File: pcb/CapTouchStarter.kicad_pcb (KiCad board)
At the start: 4 copper layers, 76.5 x 66 mm, 59 parts, among them J1 USB_C_Receptacle, J2 Conn_ARM_JTAG_SWD_10, J3 62684-50110, Q1 SS8050-G, Q2 SS8050-G, SW1 SW_SPDT, SW2 EN, SW3 BOOT, U1 CP2102N-A01-GQFN28, U2 BD48K33G-TLCT-ND, U3 ESP32-WROVER-E, U4 AMS1117-3.3

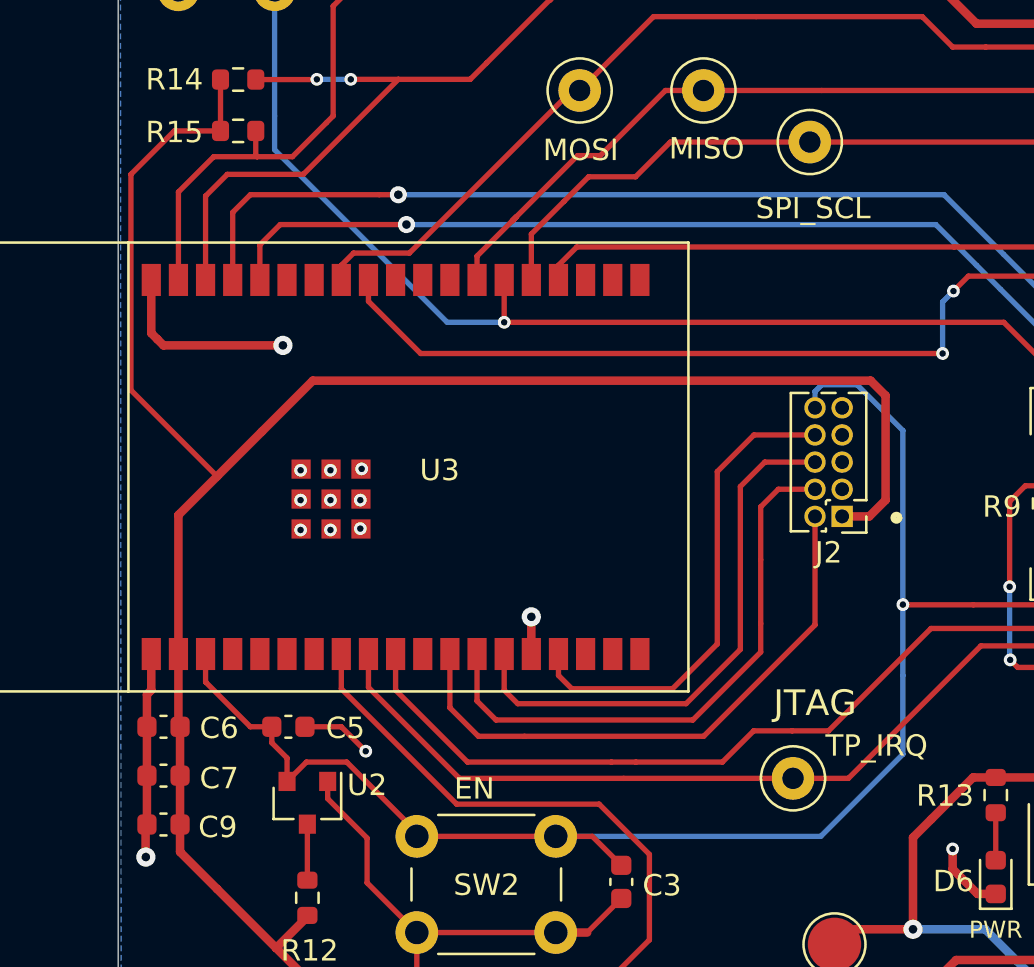
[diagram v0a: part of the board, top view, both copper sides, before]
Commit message: More DRC fixes.
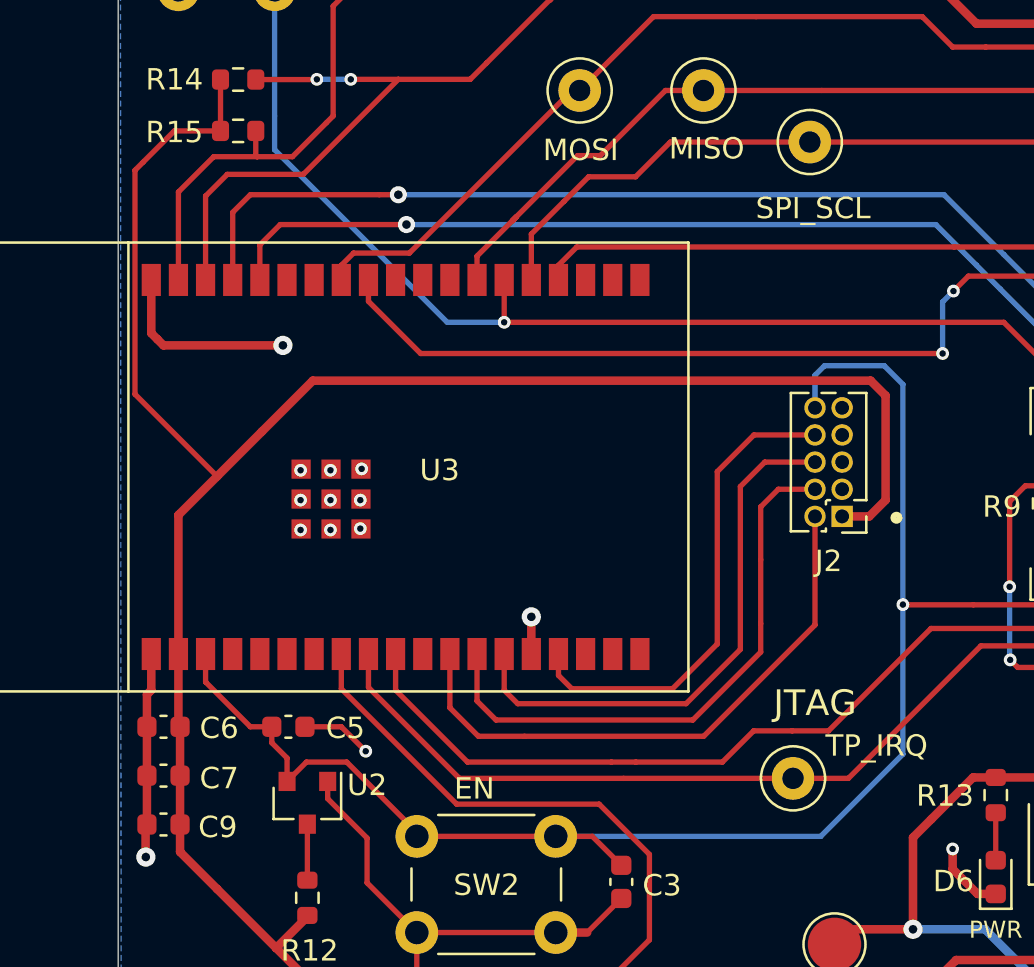
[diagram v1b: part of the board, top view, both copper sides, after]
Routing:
- net EN: track 72.7 -> 75.1 mm
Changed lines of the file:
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@@
       (effects (font (size 1 1) (thickness 0.15)))
     )
-    (fp_text value "68Ω" (at 5.842 -0.127) (layer "F.Fab")
+    (fp_text value "68Ω" (at 6.096 -0.3175) (layer "F.Fab")
       (effects (font (size 1 1) (thickness 0.15)))
     )
@@
       (effects (font (size 1 1) (thickness 0.15)))
     )
-    (fp_text value "68Ω" (at 5.842 0) (layer "F.Fab")
+    (fp_text value "68Ω" (at 6.096 -0.1905) (layer "F.Fab")
       (effects (font (size 1 1) (thickness 0.15)))
     )
@@
       (effects (font (size 1 1) (thickness 0.15)))
     )
-    (fp_text value "68Ω" (at 5.842 -0.0635) (layer "F.Fab")
+    (fp_text value "68Ω" (at 6.096 -0.254) (layer "F.Fab")
       (effects (font (size 1 1) (thickness 0.15)))
     )
@@
       (effects (font (size 1 1) (thickness 0.15)))
     )
-    (fp_text value "68Ω" (at 5.842 0) (layer "F.Fab")
+    (fp_text value "68Ω" (at 6.096 -0.1905) (layer "F.Fab")
       (effects (font (size 1 1) (thickness 0.15)))
     )
@@
       (effects (font (size 1 1) (thickness 0.15)))
     )
-    (fp_text value "BD48K33G-TLCT-ND" (at 4.064 -0.8255 180) (layer "F.Fab")
-      (effects (font (size 1 1) (thickness 0.15)))
+    (fp_text value "BD48K33G-TLCT-ND" (at 2.159 -0.0635 180) (layer "F.Fab")
+      (effects (font (size 0.3 0.3) (thickness 0.075)))
     )
     (fp_text user "${REFERENCE}" (at 0 0) (layer "F.Fab")
@@
     (tags "Through hole pin header THT 2x05 1.27mm double row")
     (attr through_hole)
-    (fp_text reference "J2" (at 0.635 -1.695) (layer "F.SilkS")
+    (fp_text reference "J2" (at 0.635 -2.0955) (layer "F.SilkS")
       (effects (font (size 1 1) (thickness 0.15)))
     )
@@
       (effects (font (size 1 1) (thickness 0.15)))
     )
-    (fp_text user "${REFERENCE}" (at 0.635 2.54 90) (layer "F.Fab")
+    (fp_text user "${REFERENCE}" (at 3.8735 4.7625 180) (layer "F.Fab")
       (effects (font (size 1 1) (thickness 0.15)))
     )
@@
   (segment (start 133.287 94.05366) (end 133.287 96.4565) (width 0.25) (layer "F.Cu") (net 2))
   (segment (start 191.246 123.53468) (end 192.21196 124.50064) (width 0.2) (layer "F.Cu") (net 2))
-  (segment (start 129.0955 98.4885) (end 131.1275 96.4565) (width 0.25) (layer "F.Cu") (net 2))
   (segment (start 175.7652 88.6488) (end 175.7652 84.8332) (width 0.25) (layer "F.Cu") (net 2))
   (segment (start 163.259 87.9475) (end 163.259 88.075) (width 0.25) (layer "F.Cu") (net 2))
@@
   (segment (start 131.3945 128.8415) (end 131.331 128.905) (width 0.4) (layer "F.Cu") (net 2))
   (segment (start 172.22256 135.24484) (end 174.51324 132.95416) (width 0.4) (layer "F.Cu") (net 2))
+  (segment (start 129.286 98.298) (end 129.667 97.917) (width 0.25) (layer "F.Cu") (net 2))
   (segment (start 199.55764 119.14632) (end 199.55764 121.64568) (width 0.4) (layer "F.Cu") (net 2))
   (segment (start 131.3945 126.619) (end 131.3945 128.8415) (width 0.4) (layer "F.Cu") (net 2))
@@
   (segment (start 191.7652 83.4202) (end 191.7652 84.0692) (width 0.25) (layer "F.Cu") (net 2))
   (segment (start 199.55764 109.28096) (end 199.55764 95.631) (width 0.4) (layer "F.Cu") (net 2))
+  (segment (start 129.286 108.7755) (end 129.286 98.298) (width 0.25) (layer "F.Cu") (net 2))
   (segment (start 141.37894 140.17244) (end 149.12594 140.17244) (width 0.4) (layer "F.Cu") (net 2))
   (segment (start 157.15996 140.19276) (end 162.75304 140.19276) (width 0.4) (layer "F.Cu") (net 2))
@@
   (segment (start 131.3945 128.905) (end 131.3945 130.188) (width 0.4) (layer "F.Cu") (net 2))
   (segment (start 131.318 114.427) (end 131.318 120.9291) (width 0.4) (layer "F.Cu") (net 2))
-  (segment (start 133.12775 112.61725) (end 129.0955 108.585) (width 0.25) (layer "F.Cu") (net 2))
   (segment (start 175.2652 83.4202) (end 175.2652 84.0792) (width 0.25) (layer "F.Cu") (net 2))
   (segment (start 199.55764 95.631) (end 197.47484 93.5482) (width 0.4) (layer "F.Cu") (net 2))
@@
   (segment (start 133.12775 112.61725) (end 131.318 114.427) (width 0.4) (layer "F.Cu") (net 2))
   (segment (start 137.3505 133.223) (end 135.89 134.6835) (width 0.4) (layer "F.Cu") (net 2))
+  (segment (start 129.667 97.917) (end 131.1275 96.4565) (width 0.25) (layer "F.Cu") (net 2))
   (segment (start 199.55764 121.64568) (end 199.55764 124.08916) (width 0.4) (layer "F.Cu") (net 2))
   (segment (start 194.87896 121.64568) (end 199.55764 121.64568) (width 0.4) (layer "F.Cu") (net 2))
   (segment (start 163.6395 114.4905) (end 164.4015 113.7285) (width 0.4) (layer "F.Cu") (net 2))
   (segment (start 199.4286 109.6142) (end 199.55764 109.74324) (width 0.25) (layer "F.Cu") (net 2))
-  (segment (start 129.0955 108.585) (end 129.0955 98.4885) (width 0.25) (layer "F.Cu") (net 2))
+  (segment (start 133.12775 112.61725) (end 129.286 108.7755) (width 0.25) (layer "F.Cu") (net 2))
   (segment (start 175.7652 83.4202) (end 175.7652 84.5792) (width 0.25) (layer "F.Cu") (net 2))
   (segment (start 163.259 82.296) (end 163.259 84.201) (width 0.6) (layer "F.Cu") (net 2))
@@
   (segment (start 139.192 125.984) (end 142.471 129.263) (width 0.25) (layer "F.Cu") (net 14))
   (via (at 165.21176 118.618) (size 0.6) (drill 0.3) (layers "F.Cu" "B.Cu") (net 14))
-  (segment (start 165.21176 110.47476) (end 165.21176 121.92508) (width 0.25) (layer "B.Cu") (net 14))
-  (segment (start 161.0995 109.4105) (end 161.0995 108.6485) (width 0.25) (layer "B.Cu") (net 14))
-  (segment (start 163.068 108.331) (end 165.21176 110.47476) (width 0.25) (layer "B.Cu") (net 14))
-  (segment (start 148.971 129.4596) (end 161.3704 129.4596) (width 0.25) (layer "B.Cu") (net 14))
-  (segment (start 161.417 108.331) (end 163.068 108.331) (width 0.25) (layer "B.Cu") (net 14))
-  (segment (start 161.0995 108.6485) (end 161.417 108.331) (width 0.25) (layer "B.Cu") (net 14))
-  (segment (start 161.3704 129.4596) (end 165.21176 125.61824) (width 0.25) (layer "B.Cu") (net 14))
-  (segment (start 165.21176 125.61824) (end 165.21176 121.92508) (width 0.25) (layer "B.Cu") (net 14))
+  (segment (start 165.21176 108.31576) (end 165.21176 125.61824) (width 0.25) (layer "B.Cu") (net 14))
+  (segment (start 164.338 107.442) (end 165.21176 108.31576) (width 0.25) (layer "B.Cu") (net 14))
+  (segment (start 161.544 107.442) (end 164.338 107.442) (width 0.25) (layer "B.Cu") (net 14))
+  (segment (start 165.21176 125.61824) (end 161.3704 129.4596) (width 0.25) (layer "B.Cu") (net 14))
+  (segment (start 161.3704 129.4596) (end 148.971 129.4596) (width 0.25) (layer "B.Cu") (net 14))
+  (segment (start 161.0995 107.8865) (end 161.544 107.442) (width 0.25) (layer "B.Cu") (net 14))
+  (segment (start 161.0995 109.4105) (end 161.0995 107.8865) (width 0.25) (layer "B.Cu") (net 14))
   (segment (start 190.22166 131.81612) (end 189.92166 131.51612) (width 0.2) (layer "F.Cu") (net 15))
   (segment (start 190.19666 133.73512) (end 190.19666 133.210119) (width 0.2) (layer "F.Cu") (net 15))
